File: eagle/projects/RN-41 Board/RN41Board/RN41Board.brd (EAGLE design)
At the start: 37.8 x 23.6 mm, 17 parts, among them J1 640456-5, Q1 MOSFET-NCHANNELSMD, U1 BLUETOOTH-RN41, U3 3.3V

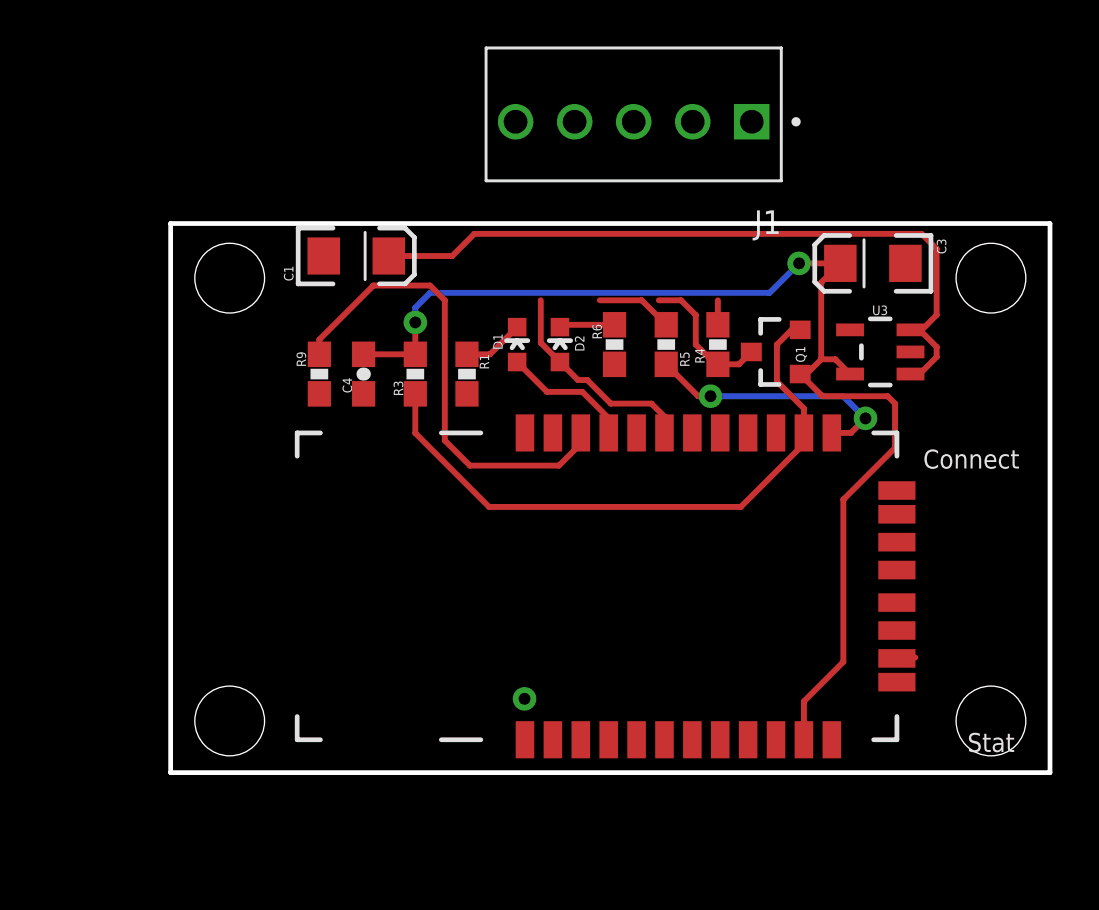
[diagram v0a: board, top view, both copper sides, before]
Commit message: RN41 Update
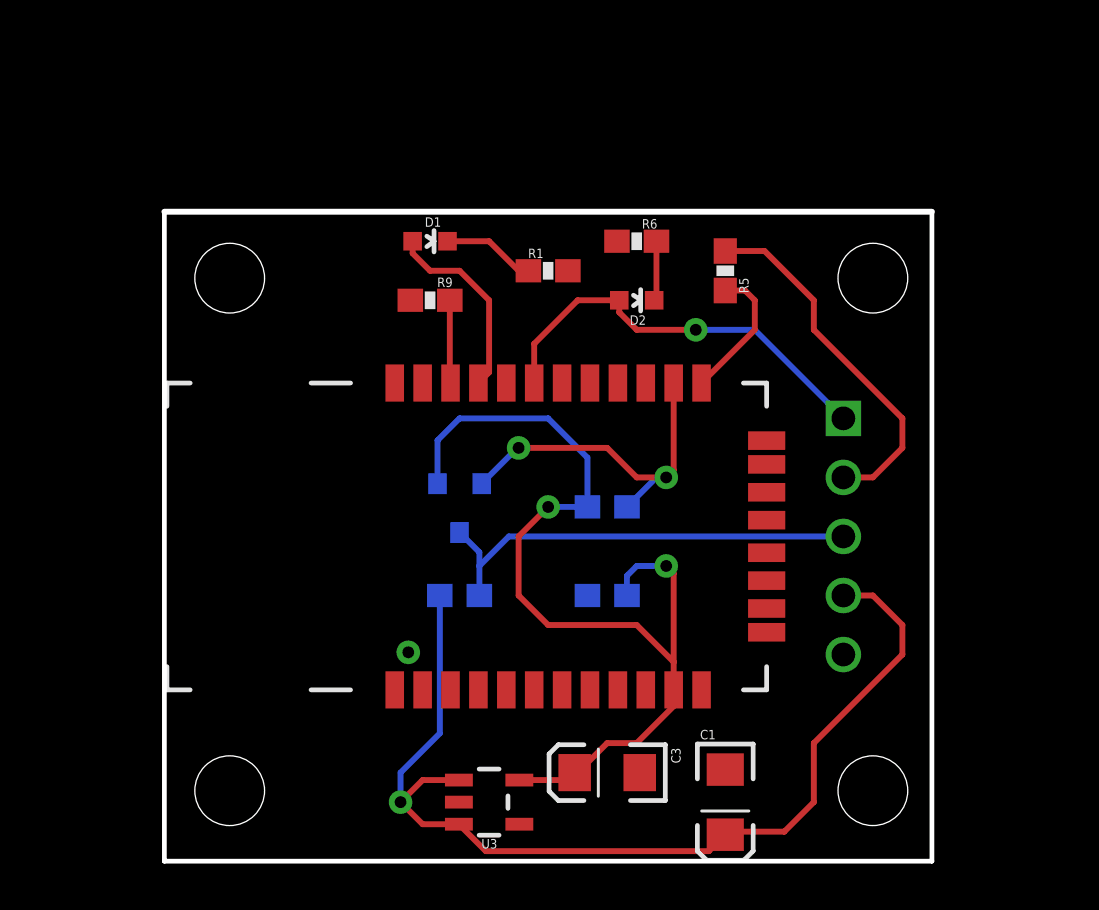
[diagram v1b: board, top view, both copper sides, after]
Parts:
- moved U$2 49.8 mm to (-30.4, 18.7)
- moved C1 28.4 mm to (22.9, -1.27), turned to 270 degrees
- moved U3 25.7 mm to (12.7, -1.27), turned to 270 degrees
- moved C3 24.7 mm to (17.8, 0.00)
- moved R4 15.5 mm to (11.4, 7.62), flipped to the bottom, turned to 180 degrees
- moved Q1 15.2 mm to (11.4, 11.4), flipped to the bottom, turned to 180 degrees
- moved C4 14.2 mm to (17.8, 7.62), flipped to the bottom, turned to 0 degrees
- moved J1 13.4 mm to (27.9, 15.2), flipped to the bottom, turned to 270 degrees
- moved R3 10.0 mm to (17.8, 11.4), flipped to the bottom, turned to 180 degrees
- moved U1 6.00 mm to (15.2, 10.2)
- moved D1 5.81 mm to (10.2, 22.9), turned to 270 degrees
- moved R9 5.72 mm to (10.2, 20.3), turned to 0 degrees
- moved R1 5.65 mm to (15.2, 21.6), turned to 0 degrees
- moved FRAME1 5.39 mm to (-0.98, 4.22)
- moved R6 4.55 mm to (19.1, 22.9), turned to 180 degrees
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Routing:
- net PIO4: track 20.4 -> 4.04 mm
- net TX_5V: track 6.09 -> 19.2 mm
- net RX_5V: track 3.29 -> 15.7 mm
- net VCC: track 32.8 -> 44.4 mm, vias 0 -> 1
- net TX: track 26.9 -> 15.5 mm, vias 0 -> 2
- net PIO2: track 9.17 -> 18.2 mm, vias 0 -> 1
- net 3.3V: track 51.1 -> 42.2 mm
- net RX: track 11.7 -> 6.42 mm, vias 2 -> 0
- net N$1: track 5.57 -> 9.03 mm
- net D1: track 2.64 -> 4.01 mm
- net GND: track 0.81 -> 0.06 mm
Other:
- board size 37.8 x 23.6 mm -> 33 x 27.9 mm
- board text removed: "Connect"
- board text removed: "Stat"

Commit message: Update RN41
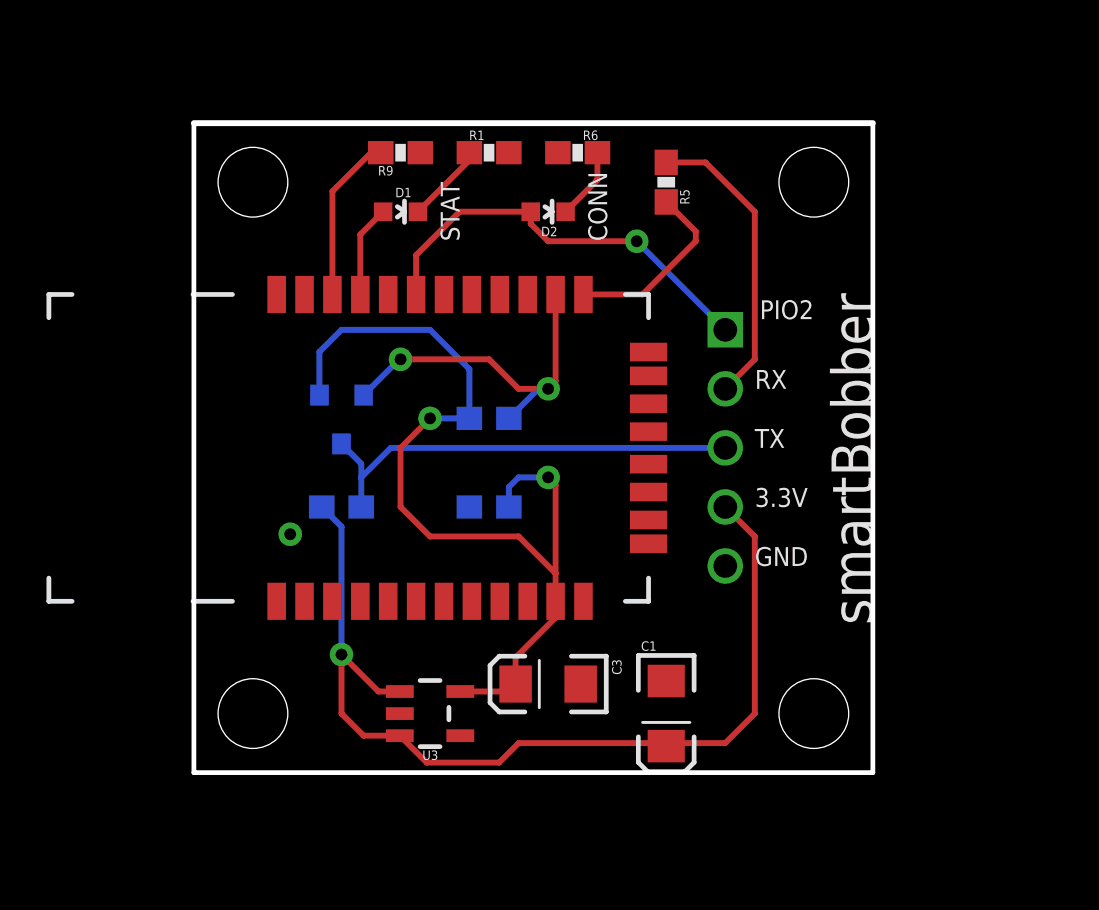
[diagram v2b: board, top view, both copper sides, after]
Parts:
- removed U$2: REVISION, SparkFun-Aesthetics:REVISION
- moved R9 6.48 mm to (8.89, 26.7), turned to 180 degrees
- moved C4 6.35 mm to (12.7, 11.4)
- moved J1 6.35 mm to (22.9, 19.1)
- moved R3 6.35 mm to (12.7, 15.2)
- moved Q1 6.35 mm to (6.35, 15.2)
- moved R4 6.35 mm to (6.35, 11.4)
- moved U1 6.35 mm to (10.2, 14.0)
- moved R1 5.68 mm to (12.7, 26.7)
- moved D2 5.39 mm to (15.2, 24.1)
- moved R6 4.58 mm to (16.5, 26.7)
- moved C1 4.58 mm to (20.3, 2.54)
- moved C3 4.58 mm to (15.2, 3.81)
- moved FRAME1 4.58 mm to (-3.52, 0.41)
- moved U3 4.58 mm to (10.2, 2.54)
- moved R5 4.58 mm to (20.3, 25.4)
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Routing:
- net N$1: track 9.03 -> 4.60 mm
- net PIO4: track 4.04 -> 7.67 mm
- net RX_5V: track 15.7 -> 12.8 mm
- net VCC: track 44.4 -> 41.6 mm
- net RX: track 6.42 -> 8.46 mm
- net 3.3V: track 42.2 -> 40.4 mm
- net D1: track 4.01 -> 3.46 mm
- net D2: track 2.58 -> 3.11 mm
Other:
- board size 33 x 27.9 mm -> 29.2 x 27.9 mm
- board text added: "3.3V"
- board text added: "CONN"
- board text added: "GND"
- board text added: "PIO2"
- board text added: "RX"
- board text added: "STAT"
- board text added: "TX"
- board text added: "smartBobber"
